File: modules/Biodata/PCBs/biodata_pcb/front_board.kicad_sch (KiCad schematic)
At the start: 20 parts, among them J1 THONKICONN, J2 THONKICONN, J3 THONKICONN, J4 THONKICONN, J5 THONKICONN, J6 THONKICONN, J7 THONKICONN, J8 THONKICONN

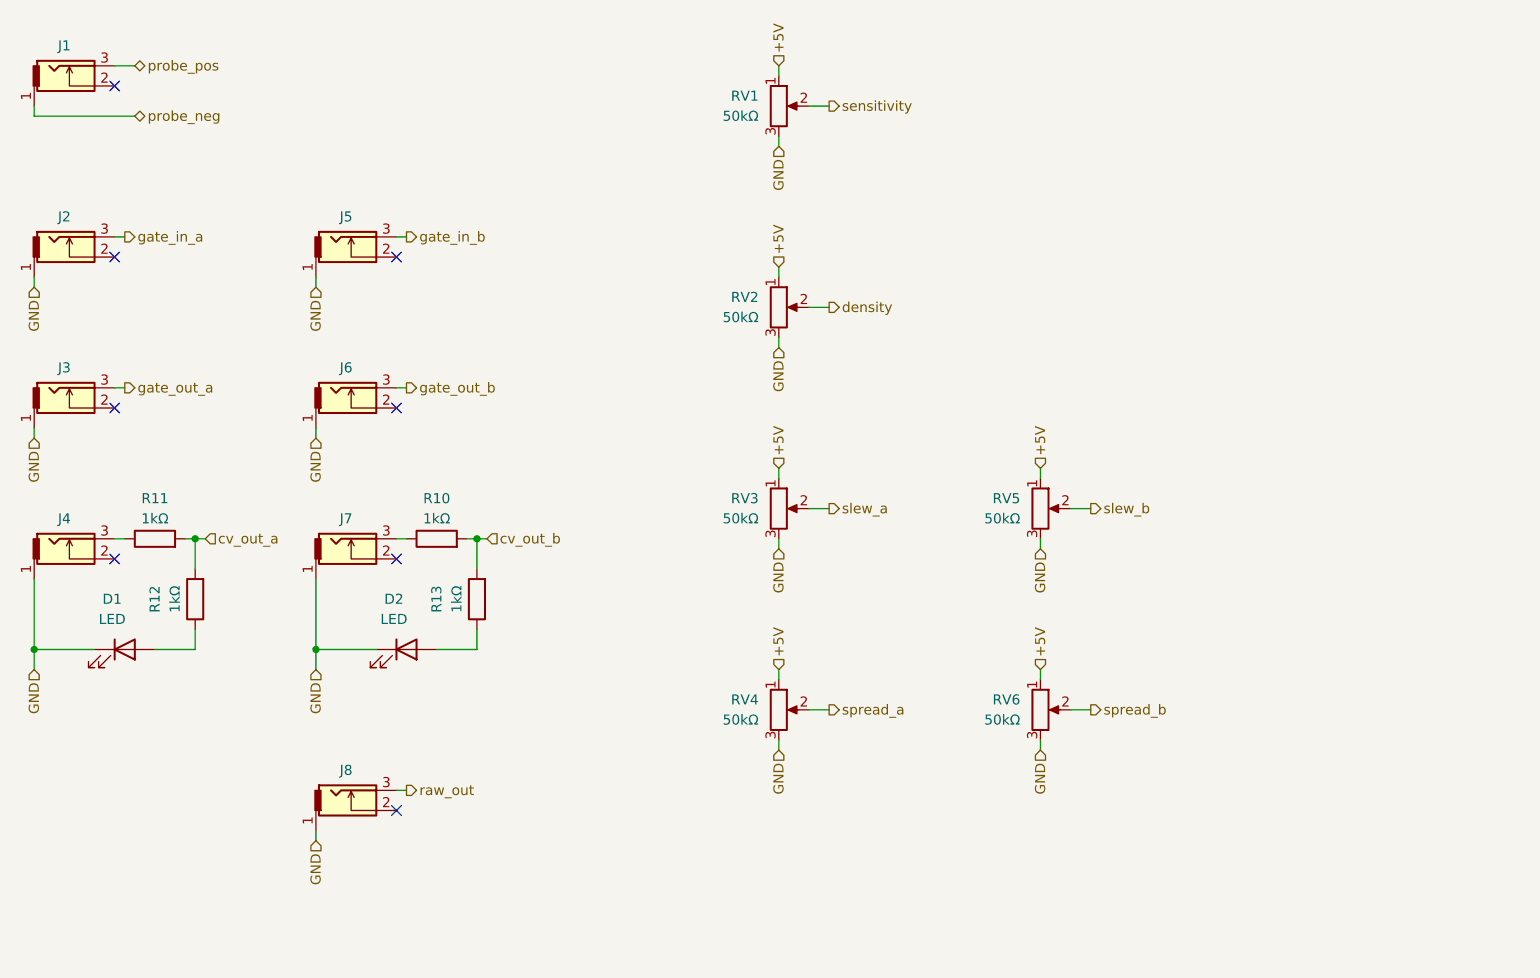
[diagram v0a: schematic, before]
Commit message: v0.1 biodata pcb
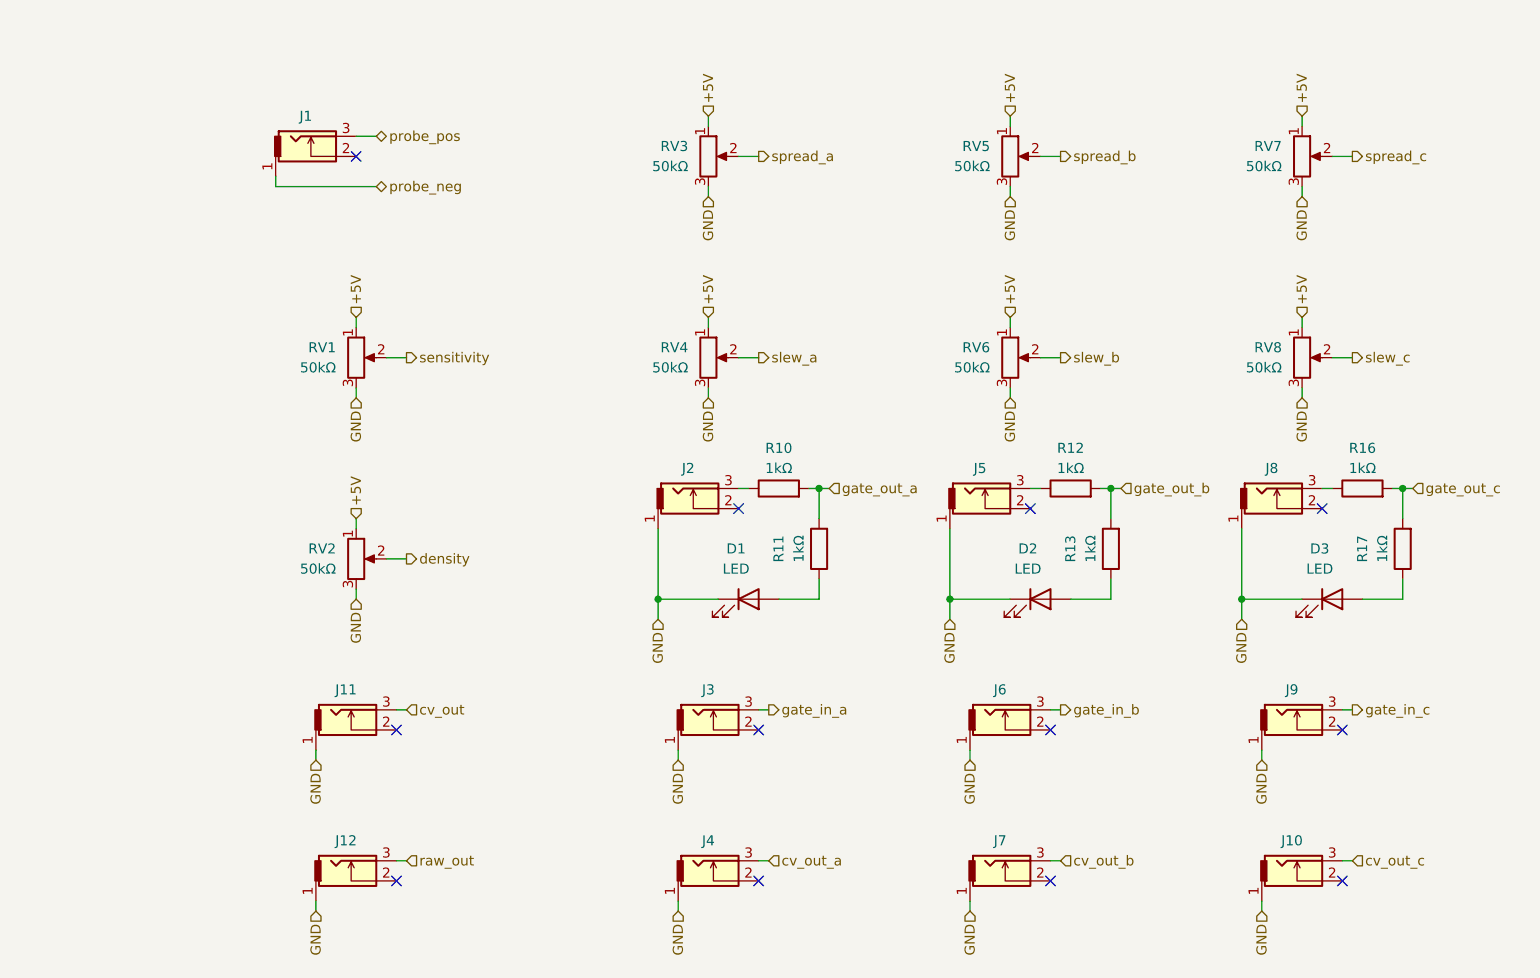
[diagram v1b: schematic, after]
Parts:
- added D3: LED, LED_THT:LED_D5.0mm, symbol Device:LED
- added J10, J12, J8, J9: THONKICONN, FreeModular:THONKICONN, symbol FreeModular:THONKICONN
- added R16, R17: 1kΩ, Resistor_THT:R_Axial_DIN0207_L6.3mm_D2.5mm_P10.16mm_Horizontal, symbol Device:R
- added RV7, RV8: 50kΩ, Potentiometer_THT:Potentiometer_Alpha_RD901F-40-00D_Single_Vertical, symbol Device:R_Potentiometer
- D1: renamed from D2; footprint (none) -> LED_THT:LED_D5.0mm
- D2: renamed from D1; footprint (none) -> LED_THT:LED_D5.0mm
- RV1, RV2, RV3, RV4, RV5, RV6: footprint (none) -> Potentiometer_THT:Potentiometer_Alpha_RD901F-40-00D_Single_Vertical
- renumbered J8 to J11, J7 to J2, J2 to J3, J3 to J4, J4 to J5, J5 to J6, J6 to J7, R13 to R11, R11 to R12, R12 to R13
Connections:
- net +5V: now also RV7.1, RV8.1
- net GND: now also D3.1 (K), J10.1, J12.1, J8.1, J9.1, RV7.3, RV8.3
- net cv_out_a: now also J4.3; no longer R12.2, R13.2
- net cv_out_b: now also J7.3; no longer R10.2, R11.2
- net gate_out_a: now also R10.2, R11.2; no longer J4.3
- net gate_out_b: now also R12.2, R13.2; no longer J7.3
- net raw_out: now also J12.3; no longer J11.3
- net slew_a: now also RV4.2; no longer RV3.2
- net slew_b: now also RV6.2; no longer RV5.2
- net spread_a: now also RV3.2; no longer RV4.2
- net spread_b: now also RV5.2; no longer RV6.2
- new net: J8.3, R16.1
- new net: D3.2 (A), R17.1
- new net cv_out: J11.3
- new net cv_out_c: J10.3
- new net gate_in_c: J9.3
- new net gate_out_c: R16.2, R17.2
- new net slew_c: RV8.2
- new net spread_c: RV7.2
- no-connect marks 8 -> 12
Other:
- company: (none) -> Free Modular
- title: (none) -> Biodata
- moved on the sheet: D1, D2, J1, J11, J2, J3, J4, J5, J6, J7, R10, R11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
